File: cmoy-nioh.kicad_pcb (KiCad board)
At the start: 2 copper layers, 72.9 x 58.6 mm, 14 parts, among them U1 OPA2604A

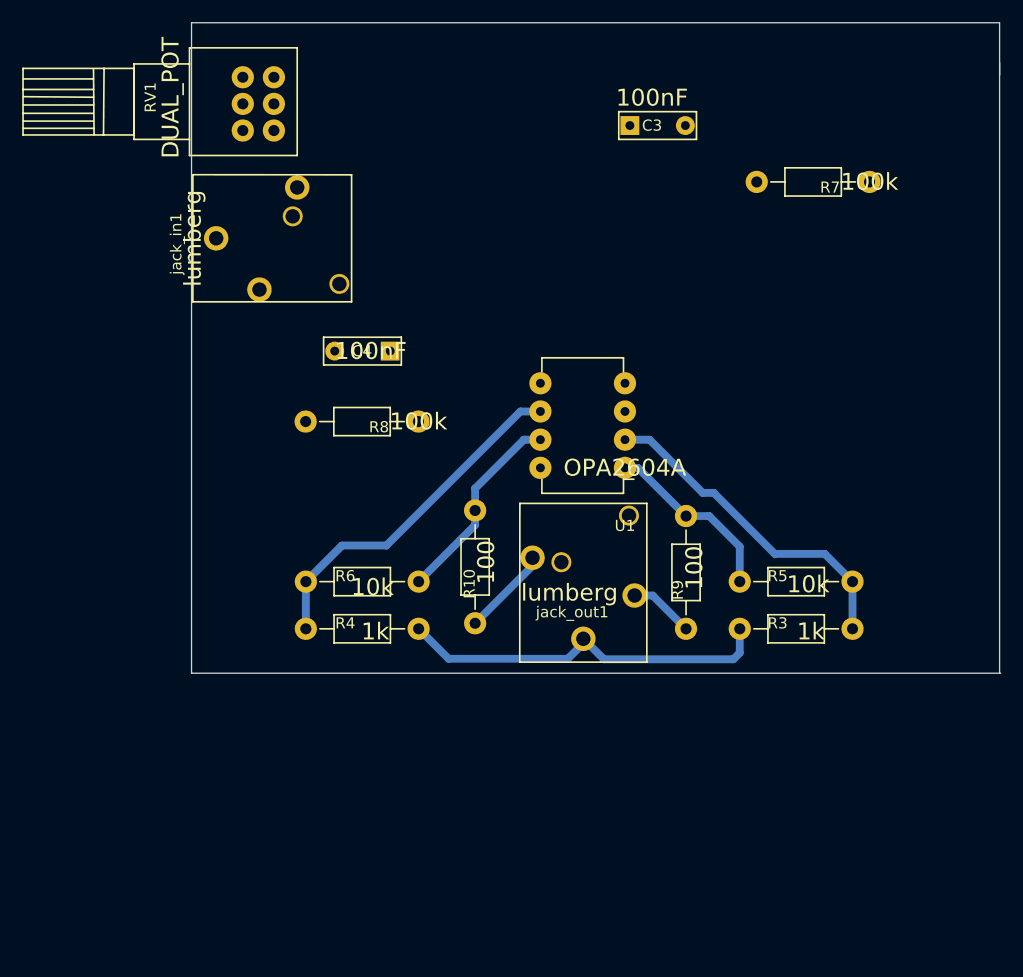
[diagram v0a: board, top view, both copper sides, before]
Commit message: dalzmian
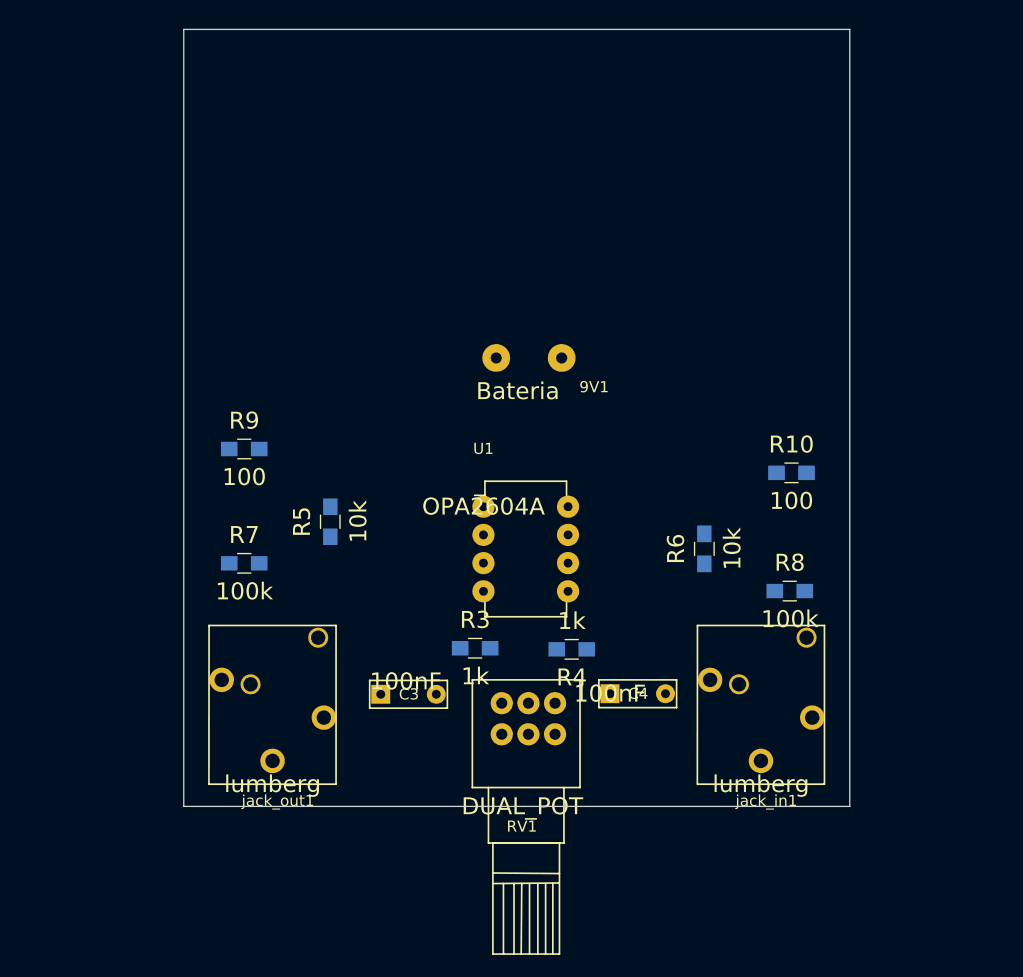
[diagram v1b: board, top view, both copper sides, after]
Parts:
- added 9V1: Bateria, tk_SolderWirePad_2x_1mmDrill-nioh, F.Cu at (114.1, 94.6)
- R10, R3, R4, R5, R6, R7, R8, R9: footprint tk_Resistor_Horizontal_RM10mm -> tk_SMD_HandSold_805_R
- moved jack_in1 71.0 mm to (135.0, 133.0), turned to 0 degrees
- moved RV1 67.5 mm to (116.0, 133.0), turned to 0 degrees
- moved R7 66.0 mm to (88.5, 113.1), turned to 0 degrees
- moved C3 55.9 mm to (100.8, 124.9)
- moved R5 47.4 mm to (96.2, 109.3), turned to 90 degrees
- moved R9 43.0 mm to (88.5, 102.8), turned to 0 degrees
- moved R8 36.8 mm to (137.6, 115.6), turned to 0 degrees
- moved C4 36.7 mm to (121.4, 124.8), turned to 0 degrees
- moved R6 36.0 mm to (129.9, 111.8), turned to 90 degrees
- moved R3 34.0 mm to (109.2, 120.8), turned to 0 degrees
- moved R10 31.6 mm to (137.8, 105.0), turned to 0 degrees
- moved jack_out1 30.1 mm to (91.0, 133.0)
- moved R4 24.0 mm to (118.0, 120.8), turned to 180 degrees
- moved U1 13.2 mm to (110.0, 108.0), turned to 0 degrees
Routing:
- net GNDREF: track 34.2 -> 0.00 mm
- net N-000003: track 31.7 -> 0.00 mm
- net N-000004: track 30.0 -> 0.00 mm
- net N-0000014: track 18.2 -> 0.00 mm
- net N-0000016: track 16.4 -> 0.00 mm
- net N-000002: track 8.04 -> 0.00 mm
- net N-0000013: track 5.87 -> 0.00 mm
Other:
- board size 72.9 x 58.6 mm -> 60 x 70 mm
